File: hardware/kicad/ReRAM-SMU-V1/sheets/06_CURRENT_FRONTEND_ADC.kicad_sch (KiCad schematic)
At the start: 21 parts, among them U11 ADA4522-2 CH1 P-leg zero-drif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, U12 ADA4522-2 CH2 N-leg (unity, r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, U13 OPA140 P-leg JFET 0.5pA *HIGH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, U14 OPA140 N-leg JFET <1pA unity, U31 ADS1262 (supply corrected: co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

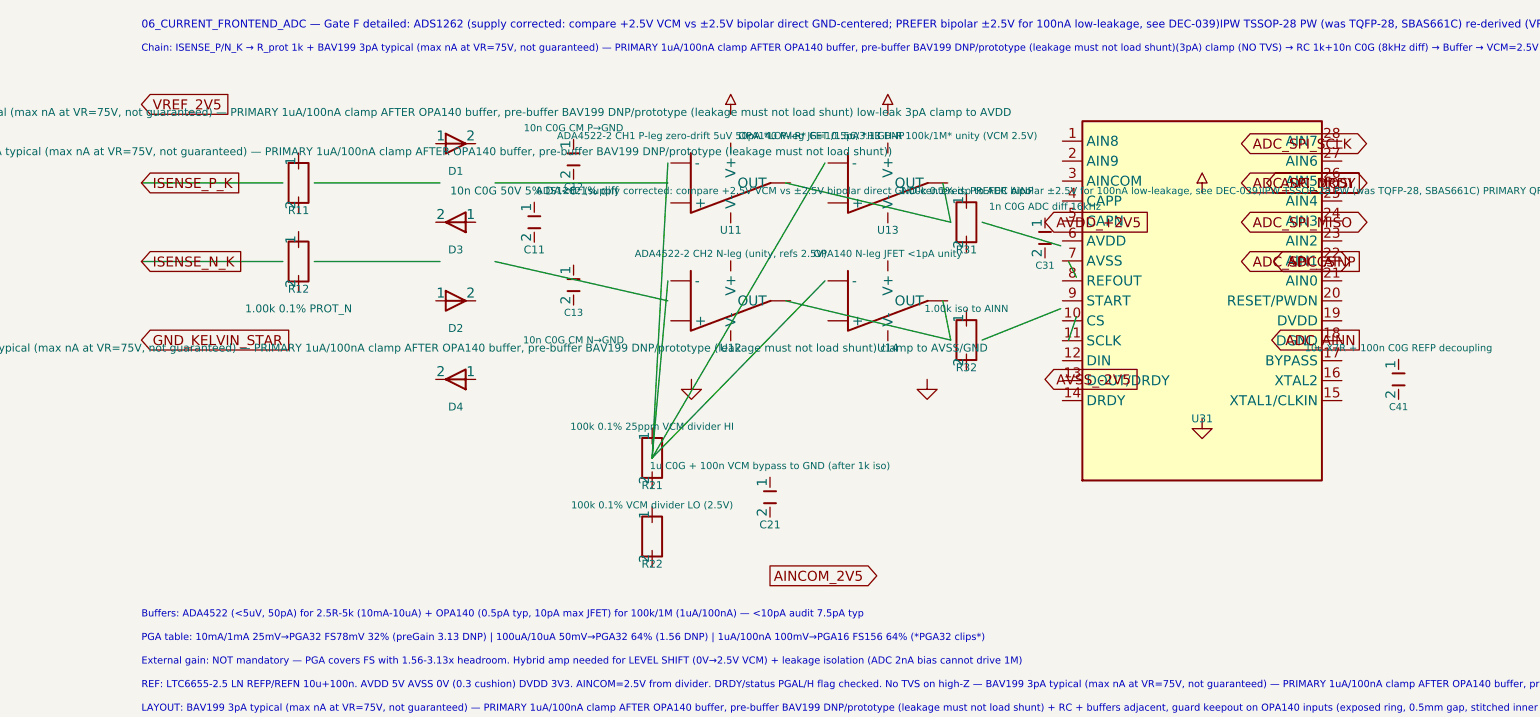
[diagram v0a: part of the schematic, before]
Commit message: Beta
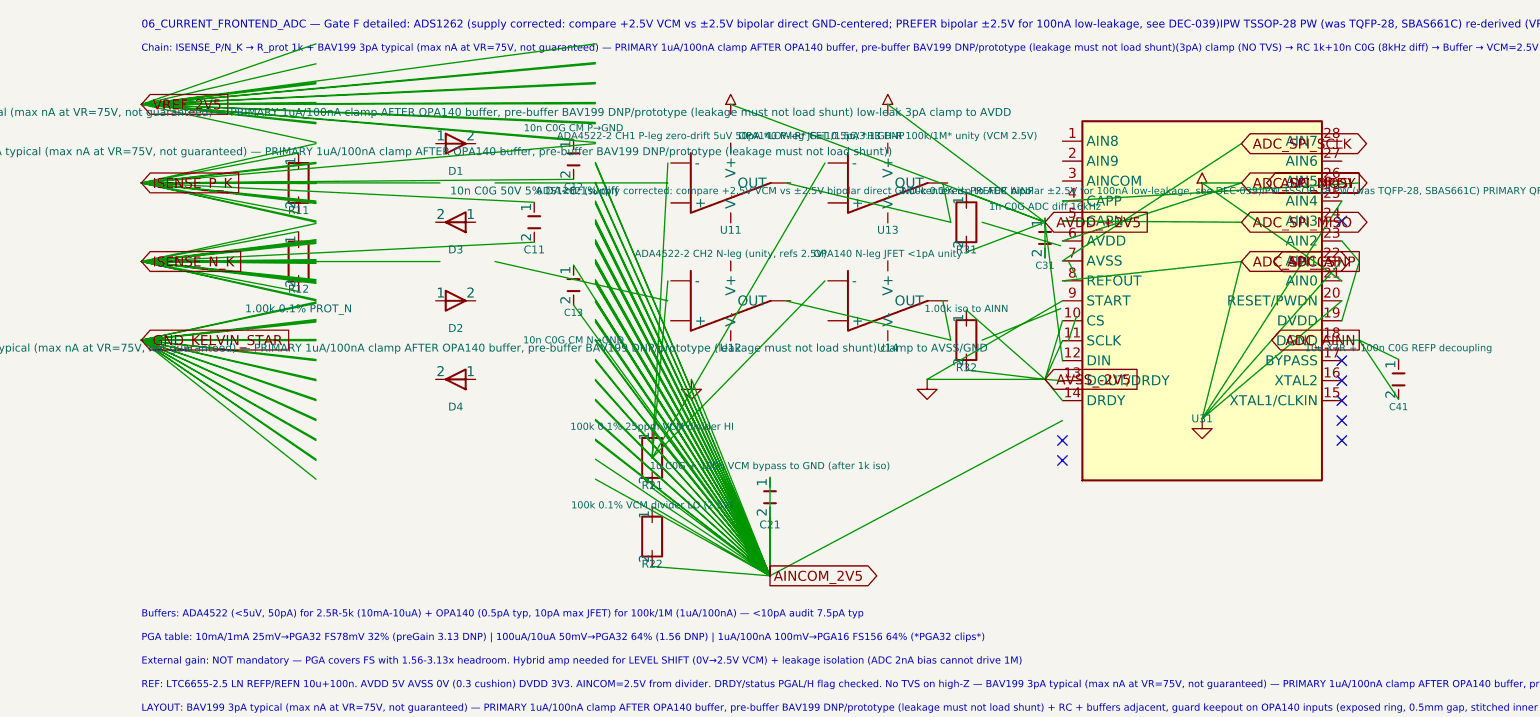
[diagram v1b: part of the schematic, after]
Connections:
- net ADC_AINN: now also C41.1, C41.2, U31.18 (DGND)
- net ADC_AINP: now also U31.19 (DVDD), U31.23 (AIN2)
- net ADC_DRDY: now also U31.4 (CAPP)
- net ADC_SPI_CS: now also U31.20 (RESET/PWDN), U31.22 (AIN1), U31.25 (AIN4), U31.8 (REFOUT)
- net ADC_SPI_MISO: now also U31.5 (CAPN)
- net ADC_SPI_MOSI: now also U31.21 (AIN0), U31.6 (AVDD)
- net ADC_SPI_SCLK: now also U31.7 (AVSS)
- net AINCOM_2V5: now also C13.1, C13.2, C21.1, C21.2, R21.1, R21.2, R22.1, R22.2
- net AVDD_+2V5: now also C31.1, C31.2, R31.1, R31.2, U31.12 (DIN)
- net AVSS_-2V5: now also R32.1, R32.2, U31.10 (CS), U31.11 (SCLK), U31.13 (DOUT/DRDY), U31.14 (DRDY), U31.9 (START)
- net ISENSE_N_K: now also C11.2, R12.1, R12.2
- net ISENSE_P_K: now also C11.1, C12.2, R11.1, R11.2
- net VREF_2V5: now also C12.1
- no-connect marks 0 -> 8
